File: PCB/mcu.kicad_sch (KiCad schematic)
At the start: 16 parts, among them J3 USB_A, SW1 SW_Push, SW2 SW_Push, SW3 SW_Push, SW4 SW_Push, U3 COM-09032, Y1 Crystal_GND24

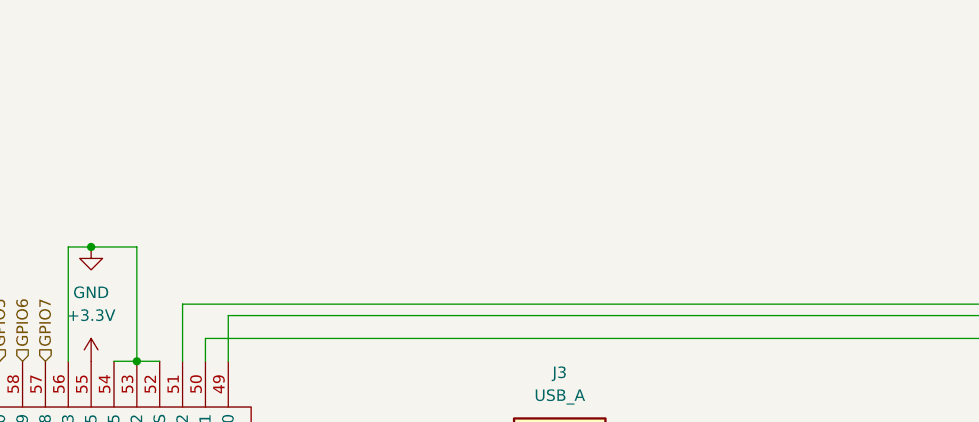
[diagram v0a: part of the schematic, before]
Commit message: pls work
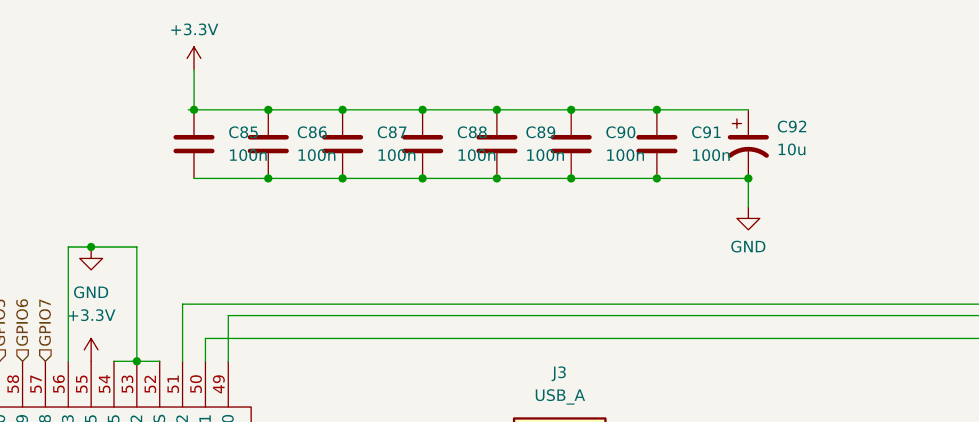
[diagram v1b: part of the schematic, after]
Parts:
- added C85, C86, C87, C88, C89, C90, C91: 100n, symbol Device:C
- added C92: 10u, symbol Device:C_Polarized_US
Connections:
- net +3.3V: now also C85.1, C86.1, C87.1, C88.1, C89.1, C90.1, C91.1, C92.1
- net GND: now also C85.2, C86.2, C87.2, C88.2, C89.2, C90.2, C91.2, C92.2

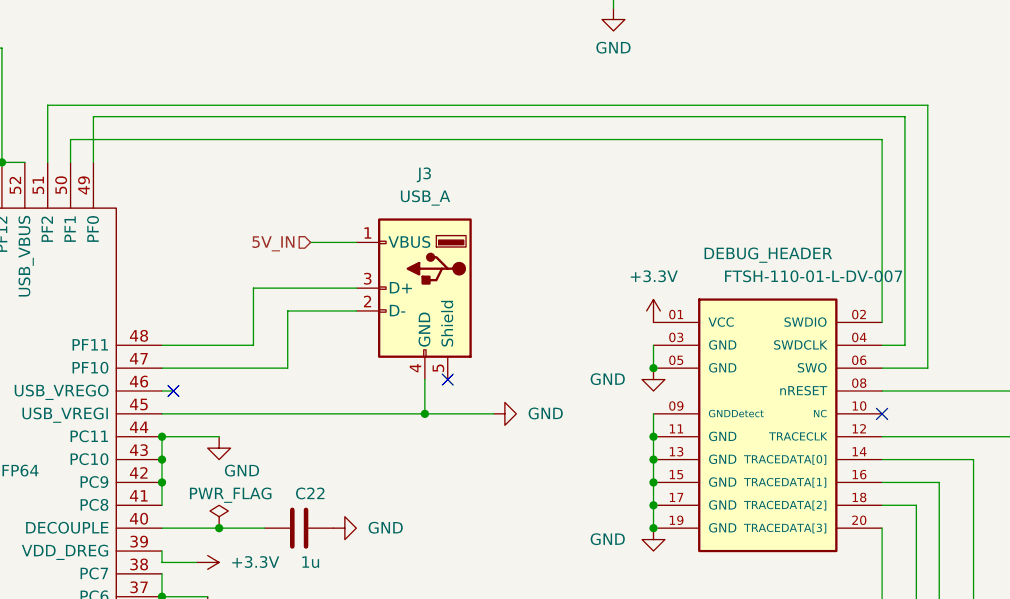
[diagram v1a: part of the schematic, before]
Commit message: Footprints
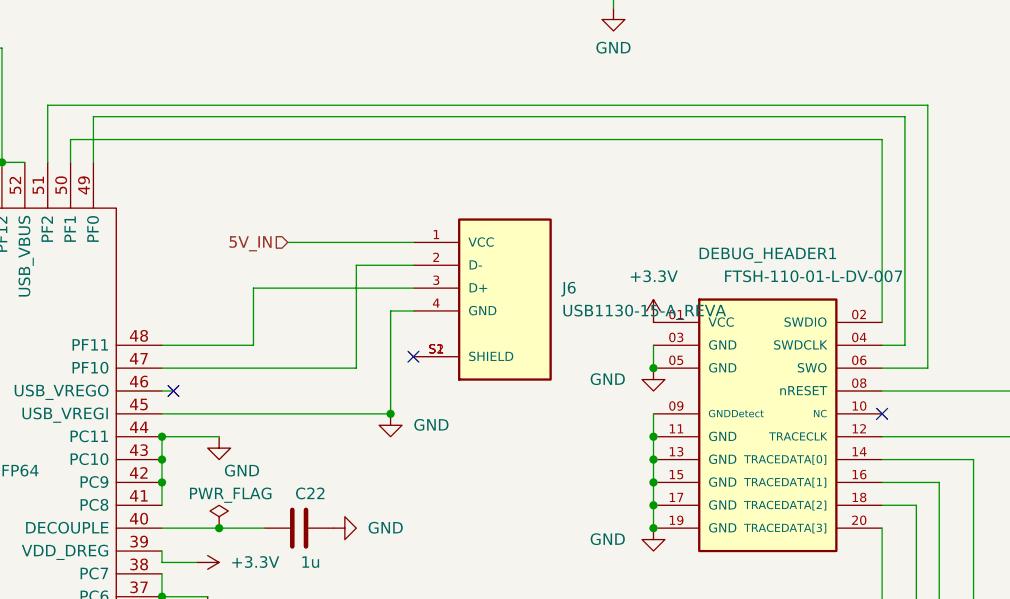
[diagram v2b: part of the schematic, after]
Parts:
- removed J3: USB_A, symbol Connector:USB_A
- added J6: USB1130-15-A_REVA, USB1130-15-A_REVA:GCT_USB1130-15-A_REVA, symbol USB1130-15-A_REVA:USB1130-15-A_REVA
- C20, C21, C22, C85, C86, C87, C88, C89, C90, C91, C92: footprint (none) -> Capacitor_SMD:C_0805_2012Metric_Pad1.18x1.45mm_HandSolder
- H1: footprint (none) -> efm32:QFP50P1200X1200X120-64N
- R10, R11, R12, R9: footprint (none) -> Resistor_SMD:R_0805_2012Metric_Pad1.20x1.40mm_HandSolder
- SW1, SW2, SW3, SW4: footprint (none) -> button:K12PBK15N
- U3: footprint COM-09032:XDCR_COM-09032 -> joystick:XDCR_COM-09032
- Y1: footprint (none) -> ECS-3953M-400-BN-TR:OSC_ECS-3953M-400-BN-TR
- renumbered DEBUG_HEADER to DEBUG_HEADER1
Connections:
- net 5V_IN: now also J6.1 (VCC)
- net GND: now also J6.4 (GND)
- net at H1.47 (PF10): now also J6.2 (D-)
- net at H1.48 (PF11): now also J6.3 (D+)
- new net: J6.S1 (SHIELD), J6.S2 (SHIELD)
